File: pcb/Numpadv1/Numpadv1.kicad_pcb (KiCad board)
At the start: 2 copper layers, 104.8 x 100 mm, 44 parts, among them J1 OLED_128x32, SW1 RotaryEncoder_Switch, SW2 Switch, SW3 Switch, SW4 Switch, U1 RP2040_Zero

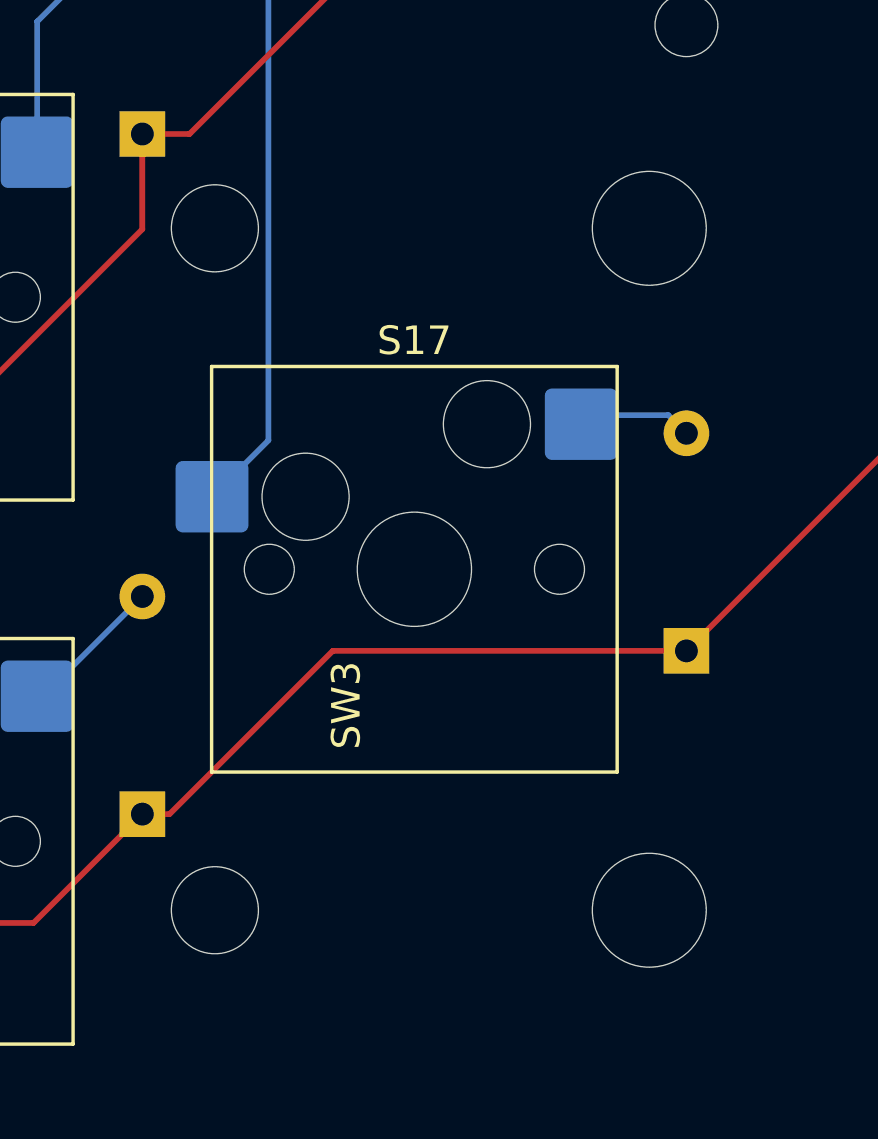
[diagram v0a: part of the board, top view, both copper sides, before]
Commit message: PCB Manufacturing Files
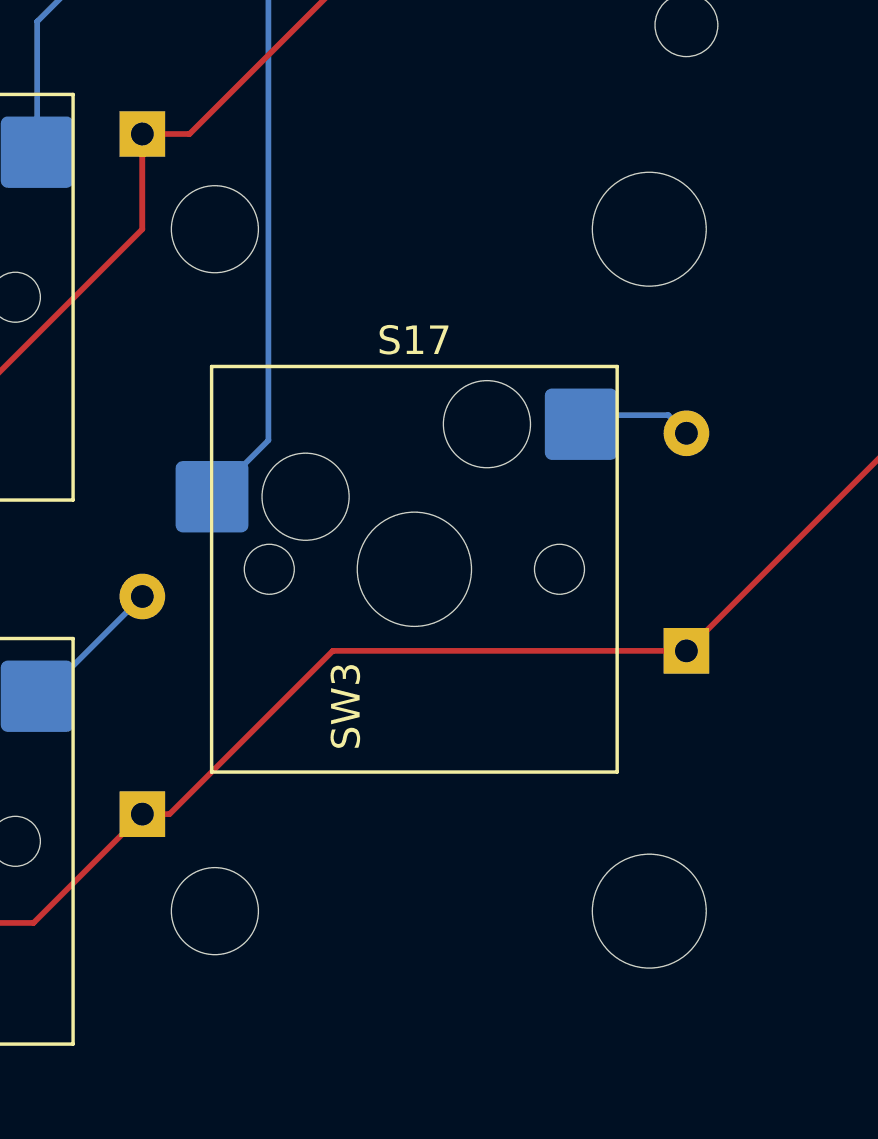
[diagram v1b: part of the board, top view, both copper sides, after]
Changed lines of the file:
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@@
 			(plot_on_all_layers_selection 0x00000000_00000000_00000000_00000000)
 			(disableapertmacros no)
-			(usegerberextensions no)
+			(usegerberextensions yes)
 			(usegerberattributes yes)
 			(usegerberadvancedattributes yes)
@@
 			(outputformat 1)
 			(mirror no)
-			(drillshape 1)
+			(drillshape 0)
 			(scaleselection 1)
-			(outputdirectory "")
+			(outputdirectory "../Fabrication/")
 		)
 	)
@@
 	(footprint "ScottoKeebs_Stabilizer:Stabilizer_MX_2.00u"
 		(layer "F.Cu")
-		(at 130.81 124.46 90)
+		(at 130.81 124.49175 90)
 		(descr "MX PCB Stabilizer 2.00u 2.25u 2.50u 2.75u")
 		(tags "MX Keyboard Stabilizer 2.00u 2.25u 2.50u 2.75u Cutout")
